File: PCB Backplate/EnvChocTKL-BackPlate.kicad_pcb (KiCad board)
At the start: 2 copper layers, 347.8 x 119.5 mm, 7 parts

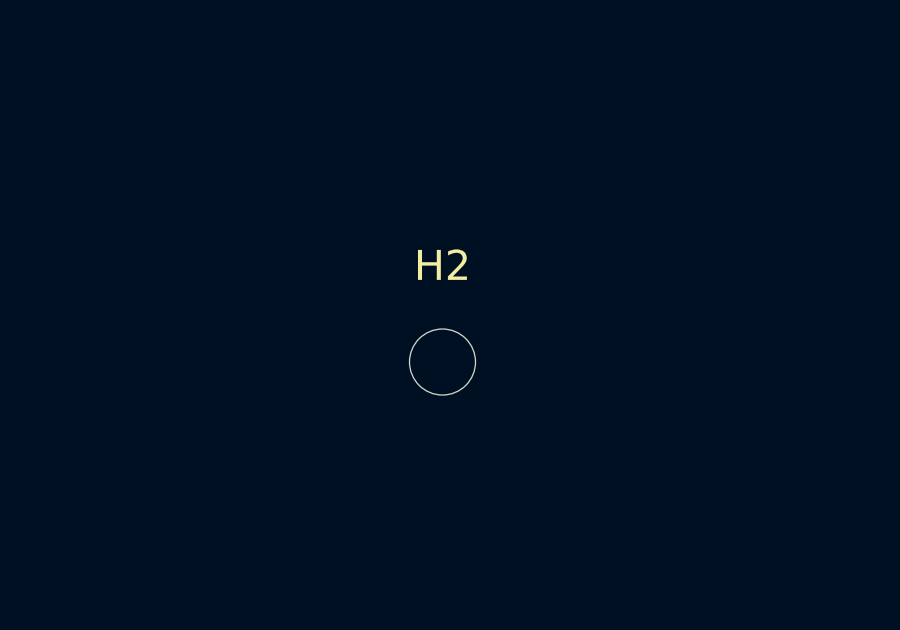
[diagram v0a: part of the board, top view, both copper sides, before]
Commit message: checks and preparation to order
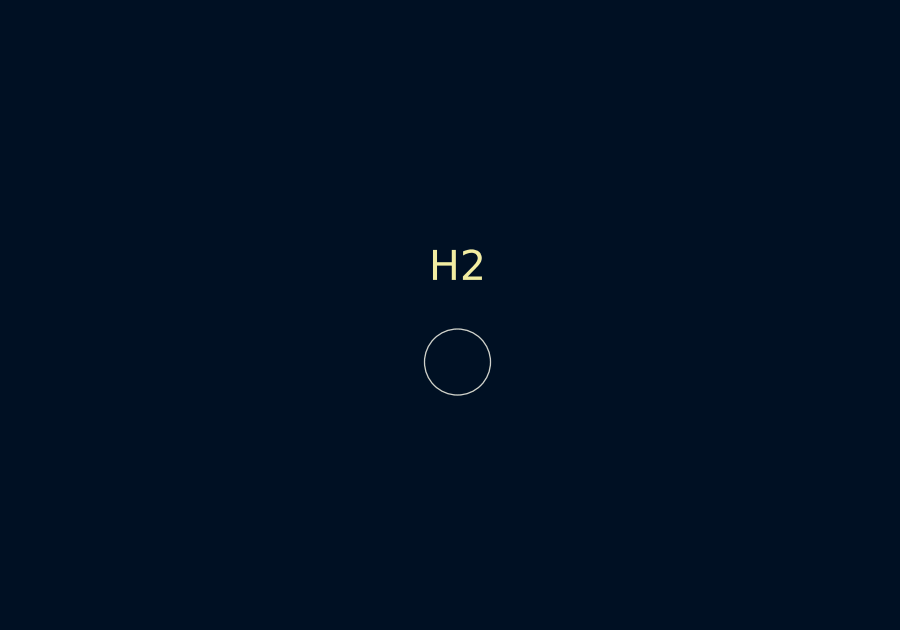
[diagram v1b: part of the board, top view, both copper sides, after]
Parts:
- moved H2 0.50 mm to (52.2, 143.9)
